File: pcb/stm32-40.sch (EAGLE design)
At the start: 83 parts, among them IC1 STM32F103RBT6, IC2 CAT24M01WI-GT3, IC3 MAX487-S, IC4 AMIS30663CANG2G, Q1 32768Hz, Q2 8MHz, SW1 KSS-2EG4430, SW2 KSS-2EG4430, X1 MCV3, X2 MCV3

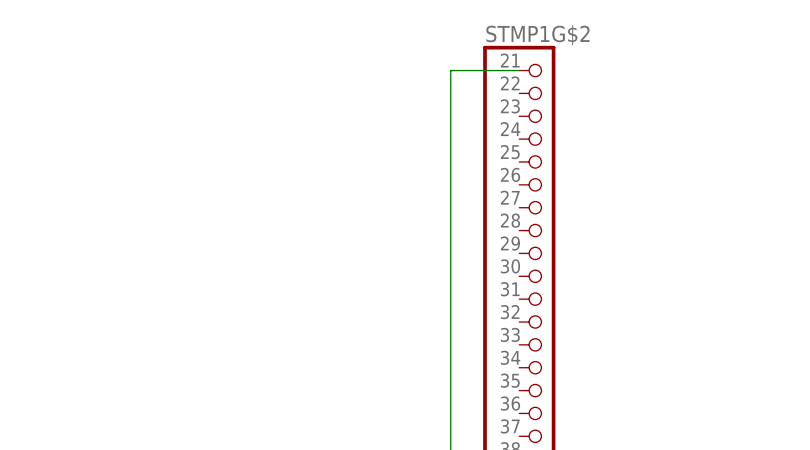
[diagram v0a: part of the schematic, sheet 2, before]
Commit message: pcb in progress
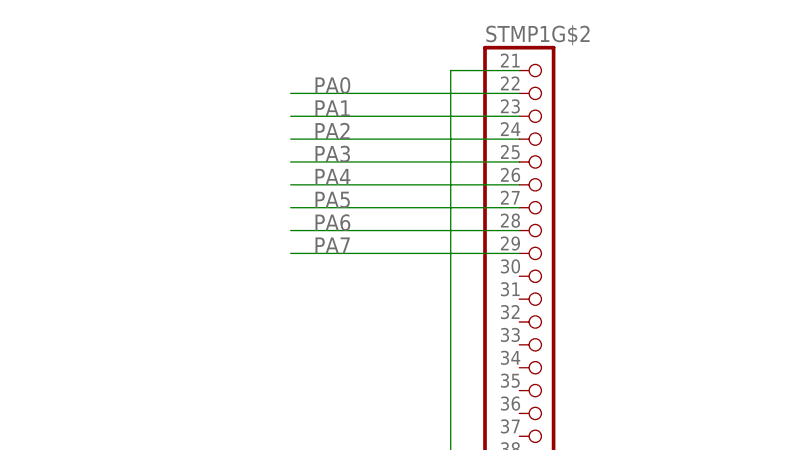
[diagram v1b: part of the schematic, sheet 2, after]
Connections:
- net PA0: now also STMP1G$2.2
- net PA1: now also STMP1G$2.3
- net PA2: now also STMP1G$2.4
- net PA3: now also STMP1G$2.5
- net PA4: now also STMP1G$2.6
- net PA5: now also STMP1G$2.7
- net PA6: now also STMP1G$2.8
- net PA7: now also STMP1G$2.9
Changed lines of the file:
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@@
+</segment>
+</net>
+<net name="PA0" class="0">
+<segment>
+<pinref part="STMP1" gate="G$2" pin="2"/>
+<wire x1="132.08" y1="226.06" x2="106.68" y2="226.06" width="0.1524" layer="91"/>
+<label x="109.22" y="226.06" size="1.778" layer="95"/>
+</segment>
+</net>
+<net name="PA1" class="0">
+<segment>
+<pinref part="STMP1" gate="G$2" pin="3"/>
+<wire x1="106.68" y1="223.52" x2="132.08" y2="223.52" width="0.1524" layer="91"/>
+<label x="109.22" y="223.52" size="1.778" layer="95"/>
+</segment>
+</net>
+<net name="PA2" class="0">
+<segment>
+<pinref part="STMP1" gate="G$2" pin="4"/>
+<wire x1="132.08" y1="220.98" x2="106.68" y2="220.98" width="0.1524" layer="91"/>
+<label x="109.22" y="220.98" size="1.778" layer="95"/>
+</segment>
+</net>
+<net name="PA3" class="0">
+<segment>
+<pinref part="STMP1" gate="G$2" pin="5"/>
+<wire x1="106.68" y1="218.44" x2="132.08" y2="218.44" width="0.1524" layer="91"/>
+<label x="109.22" y="218.44" size="1.778" layer="95"/>
+</segment>
+</net>
+<net name="PA4" class="0">
+<segment>
+<pinref part="STMP1" gate="G$2" pin="6"/>
+<wire x1="132.08" y1="215.9" x2="106.68" y2="215.9" width="0.1524" layer="91"/>
+<label x="109.22" y="215.9" size="1.778" layer="95"/>
+</segment>
+</net>
+<net name="PA5" class="0">
+<segment>
+<pinref part="STMP1" gate="G$2" pin="7"/>
+<wire x1="106.68" y1="213.36" x2="132.08" y2="213.36" width="0.1524" layer="91"/>
+<label x="109.22" y="213.36" size="1.778" layer="95"/>
+</segment>
+</net>
+<net name="PA6" class="0">
+<segment>
+<pinref part="STMP1" gate="G$2" pin="8"/>
+<wire x1="132.08" y1="210.82" x2="106.68" y2="210.82" width="0.1524" layer="91"/>
+<label x="109.22" y="210.82" size="1.778" layer="95"/>
+</segment>
+</net>
+<net name="PA7" class="0">
+<segment>
+<pinref part="STMP1" gate="G$2" pin="9"/>
+<wire x1="132.08" y1="208.28" x2="106.68" y2="208.28" width="0.1524" layer="91"/>
+<label x="109.22" y="208.28" size="1.778" layer="95"/>
 </segment>
 </net>
